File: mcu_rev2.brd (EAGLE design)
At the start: 94 x 73.3 mm, 62 parts, among them CON1 1888687, IC1 CY8C4248LQI-BL583, J1 MINIPROG3, J2 SWD, J3 90131-0937, Y1 32.768KHz, Y2 24MHz

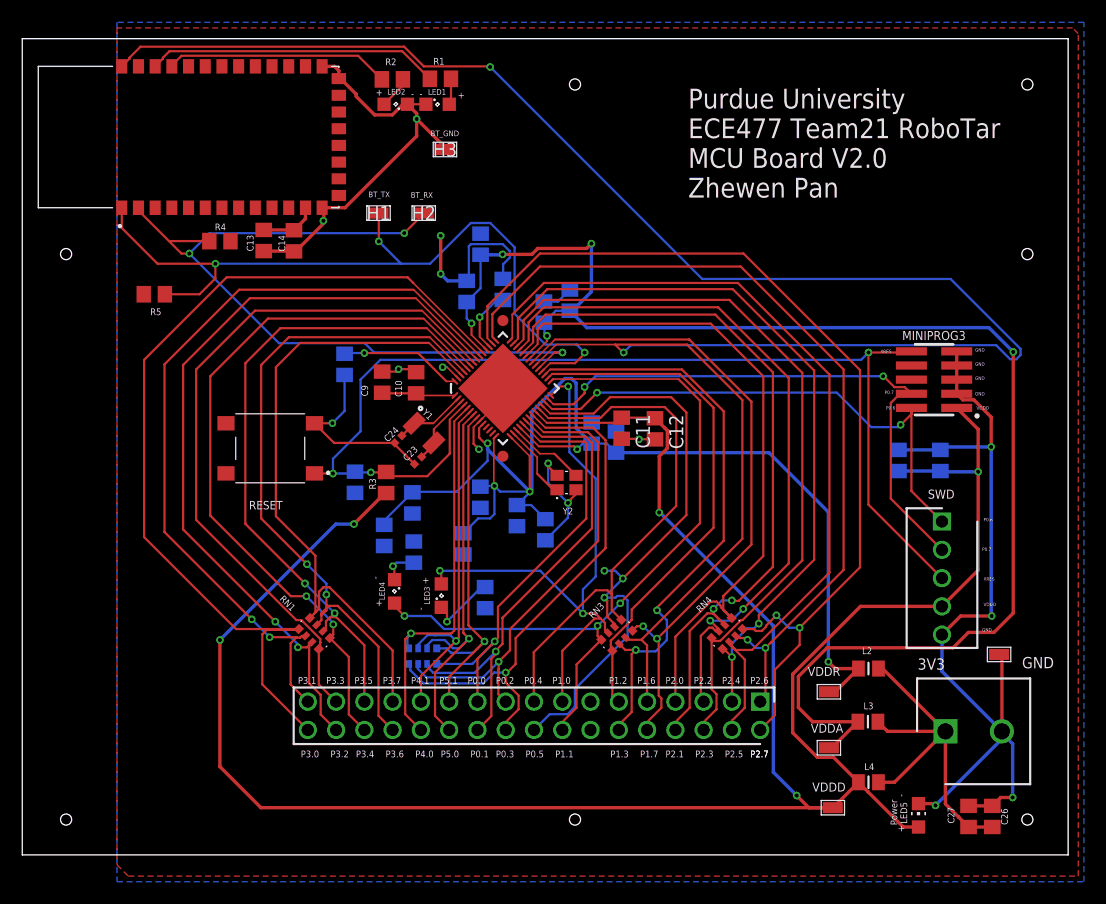
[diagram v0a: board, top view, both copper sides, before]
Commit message: ready for review and fab draft 1
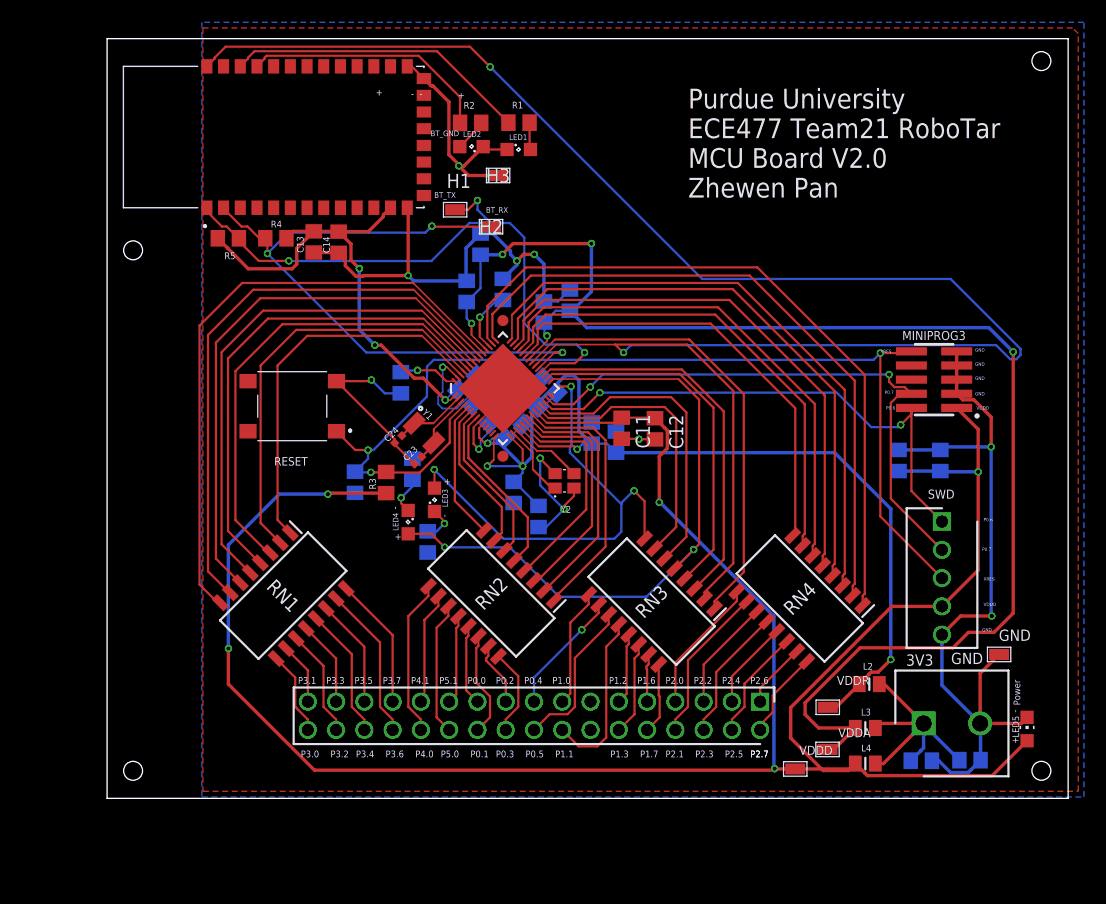
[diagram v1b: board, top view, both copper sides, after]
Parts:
- RN1, RN2, RN3, RN4: value ACASA100021000P100 -> 4816P-T01-101LF; device ACASA100021000P100:ACASA100021000P100 -> 4816P-T01-101LF:SOIC127P762X215-16N
- moved C5 20.1 mm to (61.2, 74.5), turned to 45 degrees
- moved C6 14.1 mm to (59.6, 73.3), turned to 45 degrees
- moved LED5 12.5 mm to (104.1, 43.7)
- moved C2 12.4 mm to (58.2, 71.8), turned to 45 degrees
- moved LED3 8.63 mm to (50.9, 64.3)
- moved RN2 8.36 mm to (56.0, 55.9), flipped to the top, turned to 225 degrees
- moved LED1 8.35 mm to (58.4, 95.8)
- moved R5 8.34 mm to (32.4, 87.8)
- moved R1 8.08 mm to (58.5, 98.2)
- moved R2 8.05 mm to (54.1, 98.1)
- moved LED2 7.80 mm to (54.2, 96.0)
- moved BT_SLAVE 7.65 mm to (36.8, 96.9)
- moved C9 7.59 mm to (53.6, 73.5), flipped to the bottom, turned to 225 degrees
- moved R11 7.44 mm to (48.9, 67.0)
- moved RN4 7.25 mm to (83.7, 55.4)
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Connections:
- new net P0.0_O: J3.21, RN2.13
- new net P0.1_O: J3.22, RN2.14
- new net P0.2_O: J3.19, RN2.15
- new net P0.3_O: J3.20, RN2.16
- new net P0.4_O: J3.17, RN3.10
- new net P0.5_O: J3.18, RN3.11
- new net P1.0_O: J3.15, RN3.9
- new net P1.1_O: J3.16, RN3.12
- new net P1.2_O: J3.11, RN3.13
- new net P1.3_O: J3.12, RN3.14
- new net P1.6_O: J3.9, RN3.15
- new net P1.7_O: J3.10, RN3.16
- new net P2.0_O: J3.7, RN4.9
- new net P2.1_O: J3.8, RN4.10
- new net P2.2_O: J3.5, RN4.11
- new net P2.3_O: J3.6, RN4.12
- new net P2.4_O: J3.3, RN4.13
- new net P2.5_O: J3.4, RN4.14
- new net P2.6_O: J3.1, RN4.15
- new net P2.7_O: J3.2, RN4.16
- new net P3.0_O: J3.34, RN1.9
- new net P3.1_O: J3.33, RN1.10
- new net P3.2_O: J3.32, RN1.11
- new net P3.3_O: J3.31, RN1.12
- new net P3.4_O: J3.30, RN1.13
- new net P3.5_O: J3.29, RN1.14
- new net P3.6_O: J3.28, RN1.15
- new net P3.7_O: J3.27, RN1.16
- new net P4.0_O: J3.26, RN2.9
- new net P4.1_O: J3.25, RN2.10
- new net P5.0_O: J3.24, RN2.11
- new net P5.1_O: J3.23, RN2.12
- net P0.0: now also RN2.4; no longer J3.21, RN2.5
- net P0.1: now also RN2.3; no longer J3.22, RN2.6
- net P0.2: now also RN2.2; no longer J3.19, RN2.7
- net P0.3: now also RN2.1; no longer J3.20, RN2.8
- net P0.4: now also RN3.7; no longer J3.17, RN3.1
- net P0.5: now also RN3.6; no longer J3.18, RN3.2
- net P1.0: now also RN3.8; no longer J3.15, RN3.3
- net P1.1: now also RN3.5; no longer J3.16, RN3.4
- net P1.2: now also RN3.4; no longer J3.11, RN3.5
- net P1.3: now also RN3.3; no longer J3.12, RN3.6
- net P1.6: now also RN3.2; no longer J3.9, RN3.7
- net P1.7: now also RN3.1; no longer J3.10, RN3.8
- net P2.0: now also RN4.8; no longer J3.7, RN4.1
- net P2.1: now also RN4.7; no longer J3.8, RN4.2
- net P2.2: now also RN4.6; no longer J3.5, RN4.3
- net P2.3: now also RN4.5; no longer J3.6, RN4.4
- net P2.4: now also RN4.4; no longer J3.3, RN4.5
- net P2.5: now also RN4.3; no longer J3.4, RN4.6
- net P2.6: now also RN4.2; no longer J3.1, RN4.7
- net P2.7: now also RN4.1; no longer J3.2, RN4.8
- net P3.0: now also RN1.8; no longer J3.34, RN1.1
- net P3.1: now also RN1.7; no longer J3.33, RN1.2
- net P3.2: now also RN1.6; no longer J3.32, RN1.3
- net P3.3: now also RN1.5; no longer J3.31, RN1.4
- net P3.4: now also RN1.4; no longer J3.30, RN1.5
- net P3.5: now also RN1.3; no longer J3.29, RN1.6
- net P3.6: now also RN1.2; no longer J3.28, RN1.7
- net P3.7: now also RN1.1; no longer J3.27, RN1.8
- net P4.0: now also RN2.8; no longer J3.26, RN2.1
- net P4.1: now also RN2.7; no longer J3.25, RN2.2
- net P5.0: now also RN2.6; no longer J3.24, RN2.3
- net P5.1: now also RN2.5; no longer J3.23, RN2.4
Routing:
- net VDDD: track 221.5 -> 255.3 mm, vias 5 -> 8
- net P0.5: track 57.5 -> 28.5 mm, vias 3 -> 0
- net P3.0: track 83.4 -> 55.5 mm
- net P0.3: track 48.4 -> 23.9 mm, vias 1 -> 0
- net P3.7: track 58.7 -> 34.6 mm
- net P3.6: track 61.8 -> 37.8 mm, vias 2 -> 0
- net P2.1: track 66.8 -> 43.7 mm, vias 2 -> 0
- net P4.0: track 35.4 -> 12.6 mm, vias 1 -> 0
- net P0.1: track 44.3 -> 21.5 mm, vias 1 -> 0
- net P0.4: track 48.4 -> 26.1 mm
- net P2.7: track 85.7 -> 63.7 mm, vias 2 -> 0
- net P1.6: track 185.0 -> 163.4 mm
- net P3.2: track 71.2 -> 49.9 mm, vias 2 -> 0
- net P3.4: track 65.9 -> 44.6 mm, vias 2 -> 0
- net P5.0: track 35.6 -> 14.8 mm, vias 1 -> 0
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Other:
- board size 94 x 73.3 mm -> 86.3 x 68.2 mm
